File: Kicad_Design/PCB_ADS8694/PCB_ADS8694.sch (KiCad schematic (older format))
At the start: 47 parts, among them J1 Screw_Terminal_01x03_Alimenta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, J2 Conn_01x06_Male, J3 Conn_01x06_Male, J5 Screw_Terminal_01x02_CH3, J6 Screw_Terminal_01x02_CH2, J7 Screw_Terminal_01x02_CH1, J8 Screw_Terminal_01x02_CH0, U1 LM7805_TO220, U2 AD8221, U3 AD8221, U4 ADS8694_Vers2, U5 AD8221, U6 AD8221

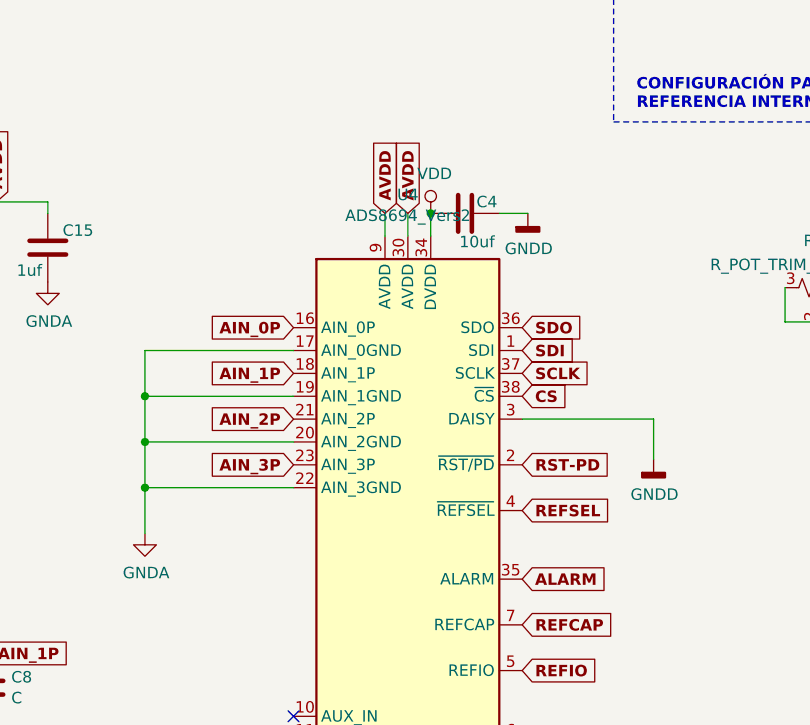
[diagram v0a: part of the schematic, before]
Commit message: version finalizada
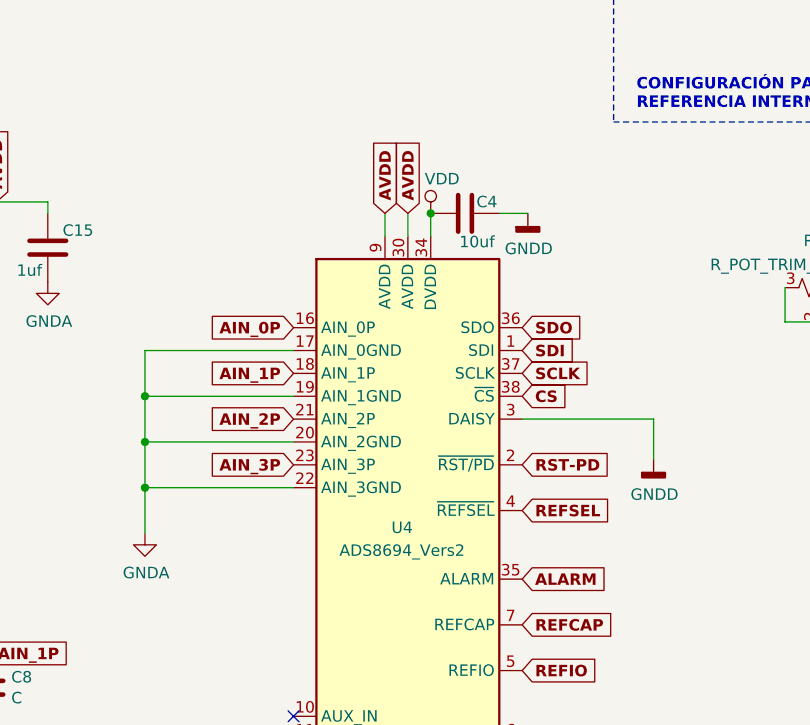
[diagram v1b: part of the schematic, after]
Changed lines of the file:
@@
 P 5850 3100
 F 0 "#PWR09" H 5850 2950 50  0001 C CNN
-F 1 "VDD" H 5867 3273 50  0000 C CNN
+F 1 "VDD" H 5900 3250 50  0000 C CNN
 F 2 "" H 5850 3100 50  0001 C CNN
 F 3 "" H 5850 3100 50  0001 C CNN
@@
 U 1 1 5CE32CBF
 P 5750 4500
-F 0 "U4" H 5750 5981 50  0000 C CNN
-F 1 "ADS8694_Vers2" H 5750 5890 50  0000 C CNN
+F 0 "U4" H 5725 4525 50  0000 C CNN
+F 1 "ADS8694_Vers2" H 5725 4425 50  0000 C CNN
 F 2 "Package_SO:TSSOP-38_4.4x9.7mm_P0.5mm" H 5750 4500 50  0001 C CNN
 F 3 "http://www.ti.com/lit/ds/symlink/ads8694.pdf" H 6700 5800 50  0001 C CNN
